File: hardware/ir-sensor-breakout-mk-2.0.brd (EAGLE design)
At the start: 24 x 29 mm, 6 parts, among them U1 MLX906145V-PTH

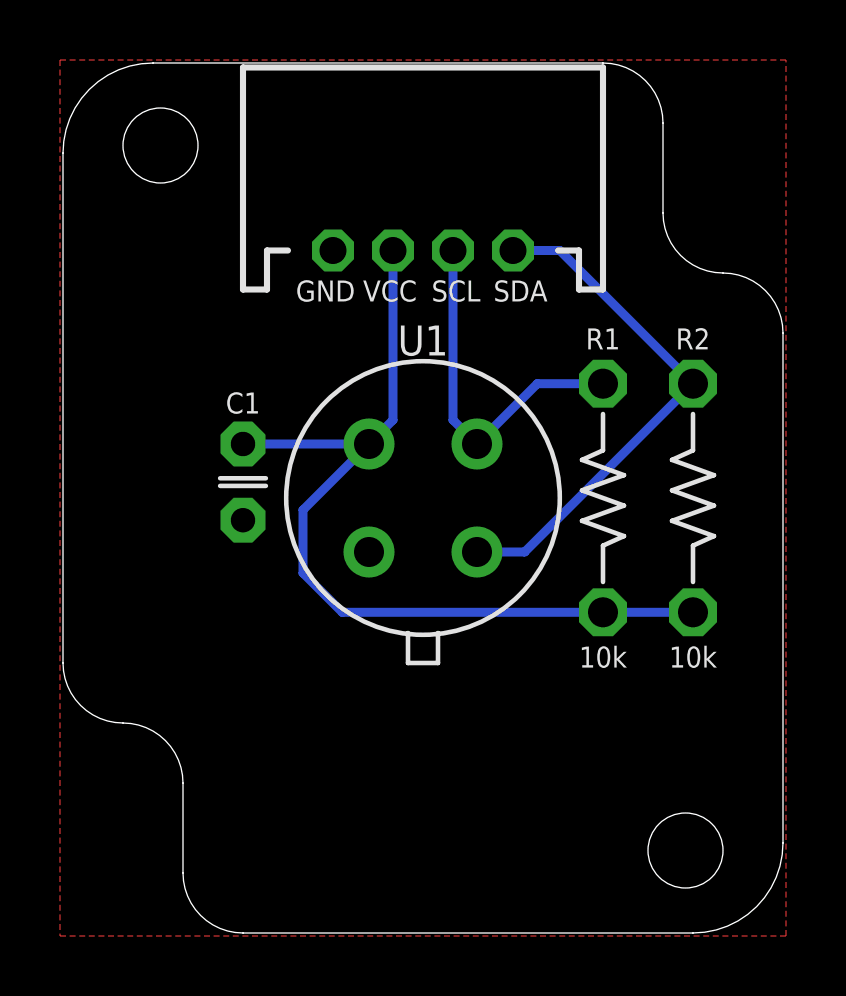
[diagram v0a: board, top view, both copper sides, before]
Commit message: twiddling around with IR sensor breakouts
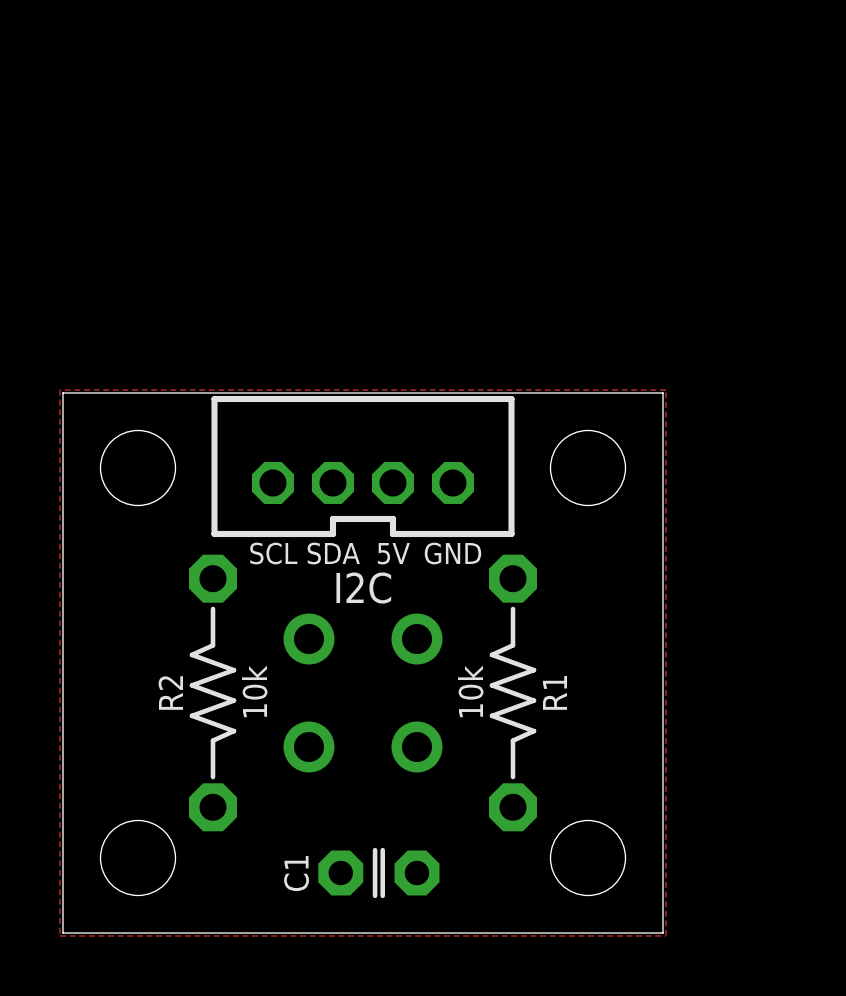
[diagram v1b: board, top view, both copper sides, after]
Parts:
- removed JP1: M04JST-PTH, A_butts:JST-4-PH-RA-PTH
- added I2C: M04JST-PTH-VERT, A_butts:JST-4-PH-VERT-PTH
- C1: value 0.1uF -> 100nF
- FRAME1: value (none) -> FRAME-LETTERNO_PACKAGE
- moved R2 17.3 mm to (5.00, 8.00)
- moved C1 13.8 mm to (10.5, 2.00), turned to 180 degrees
- moved R1 7.16 mm to (15.0, 8.00)
- moved U1 6.80 mm to (10.0, 8.00), flipped to the bottom, turned to 270 degrees
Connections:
- net GND: now also I2C.4; no longer JP1.1
- net SCL: now also I2C.1; no longer JP1.4
- net SDA: now also I2C.2; no longer JP1.3
- net VCC: now also I2C.3; no longer JP1.2
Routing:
- net VCC: track 29.7 -> 0.00 mm
- net SCL: track 17.4 -> 0.00 mm
- net SDA: track 11.8 -> 0.00 mm
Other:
- board size 24 x 29 mm -> 20 x 18 mm
- board text added: "5V"
- board text removed: "VCC"
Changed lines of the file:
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@@
 <board>
 <plain>
-<wire x1="0" y1="26" x2="0" y2="9" width="0" layer="20"/>
-<wire x1="0" y1="9" x2="2" y2="7" width="0" layer="20" curve="90"/>
-<wire x1="2" y1="7" x2="4" y2="5" width="0" layer="20" curve="-90"/>
-<wire x1="4" y1="5" x2="4" y2="2" width="0" layer="20"/>
-<wire x1="4" y1="2" x2="6" y2="0" width="0" layer="20" curve="90"/>
-<wire x1="6" y1="0" x2="21" y2="0" width="0" layer="20"/>
-<wire x1="21" y1="0" x2="24" y2="3" width="0" layer="20" curve="90"/>
-<wire x1="22" y1="22" x2="24" y2="20" width="0" layer="20" curve="-90"/>
-<wire x1="24" y1="20" x2="24" y2="3" width="0" layer="20"/>
-<wire x1="20" y1="27" x2="20" y2="24" width="0" layer="20"/>
-<wire x1="20" y1="24" x2="22" y2="22" width="0" layer="20" curve="90"/>
-<wire x1="20" y1="27" x2="18" y2="29" width="0" layer="20" curve="90"/>
-<wire x1="18" y1="29" x2="3" y2="29" width="0" layer="20"/>
-<wire x1="3" y1="29" x2="0" y2="26" width="0" layer="20" curve="90"/>
-<hole x="20.75" y="2.75" drill="2.5"/>
-<hole x="3.25" y="26.25" drill="2.5"/>
-<text x="8.75" y="21.75" size="0.7" layer="21" font="vector" ratio="12" align="top-center">GND</text>
-<text x="10.9" y="21.75" size="0.7" layer="21" font="vector" ratio="12" align="top-center">VCC</text>
-<text x="15.25" y="21.75" size="0.7" layer="21" font="vector" ratio="12" align="top-center">SDA</text>
-<text x="13.1" y="21.75" size="0.7" layer="21" font="vector" ratio="12" align="top-center">SCL</text>
-<text x="8.75" y="21.75" size="0.7" layer="22" font="vector" ratio="12" rot="MR180" align="bottom-center">GND</text>
-<text x="10.9" y="21.75" size="0.7" layer="22" font="vector" ratio="12" rot="MR180" align="bottom-center">VCC</text>
-<text x="15.25" y="21.75" size="0.7" layer="22" font="vector" ratio="12" rot="MR180" align="bottom-center">SDA</text>
-<text x="13.1" y="21.75" size="0.7" layer="22" font="vector" ratio="12" rot="MR180" align="bottom-center">SCL</text>
+<wire x1="0" y1="18" x2="0" y2="0" width="0" layer="20"/>
+<wire x1="0" y1="0" x2="20" y2="0" width="0" layer="20"/>
+<wire x1="20" y1="18" x2="20" y2="0" width="0" layer="20"/>
+<wire x1="20" y1="18" x2="0" y2="18" width="0" layer="20"/>
+<hole x="17.5" y="15.5" drill="2.5"/>
+<hole x="2.5" y="15.5" drill="2.5"/>
+<text x="13" y="13" size="0.7" layer="21" font="vector" ratio="12" align="top-center">GND</text>
+<text x="11" y="13" size="0.7" layer="21" font="vector" ratio="12" align="top-center">5V</text>
+<text x="9" y="13" size="0.7" layer="21" font="vector" ratio="12" align="top-center">SDA</text>
+<text x="7" y="13" size="0.7" layer="21" font="vector" ratio="12" align="top-center">SCL</text>
+<text x="13" y="13.5" size="0.7" layer="22" font="vector" ratio="12" rot="MR180" align="bottom-center">GND</text>
+<text x="11" y="13.5" size="0.7" layer="22" font="vector" ratio="12" rot="MR180" align="bottom-center">5V</text>
+<text x="9" y="13.5" size="0.7" layer="22" font="vector" ratio="12" rot="MR180" align="bottom-center">SDA</text>
+<text x="7" y="13.5" size="0.7" layer="22" font="vector" ratio="12" rot="MR180" align="bottom-center">SCL</text>
+<hole x="17.5" y="2.5" drill="2.5"/>
+<hole x="2.5" y="2.5" drill="2.5"/>
 </plain>
 <attributes>
@@
 </autorouter>
 <elements>
-<element name="FRAME1" library="A_butts" package="DUMMY" value="" x="0" y="0">
+<element name="FRAME1" library="A_butts" package="DUMMY" value="FRAME-LETTERNO_PACKAGE" x="0" y="0">
 <attribute name="VERSION" value="v01" x="0" y="0" size="0.5" layer="27" font="vector" ratio="12" display="off"/>
 <attribute name="DESIGNER" value="Nobody" x="0" y="0" size="0.5" layer="27" font="vector" ratio="12" display="off"/>
 </element>
-<element name="JP1" library="A_butts" package="JST-4-PH-RA-PTH" value="M04JST-PTH" x="9" y="22.75" smashed="yes">
-<attribute name="SKU" value="PRT-09916" x="9" y="22.75" size="1.778" layer="27" display="off"/>
-</element>
-<element name="U1" library="A_butts" package="TO-39-4" value="MLX906145V-PTH" x="12" y="14.5" smashed="yes" rot="R180">
-<attribute name="NAME" x="12" y="19.25" size="1" layer="25" font="vector" ratio="12" rot="R180" align="top-center"/>
-</element>
-<element name="C1" library="A_butts" package="C025-024X044" value="0.1uF" x="6" y="15.03" rot="R270"/>
-<element name="R1" library="A_butts" package="RESISTOR-AXIAL-PTH-7.62MM" value="10k" x="18" y="14.5" rot="R270"/>
-<element name="R2" library="A_butts" package="RESISTOR-AXIAL-PTH-7.62MM" value="10k" x="21" y="14.5" rot="R270"/>
+<element name="I2C" library="A_butts" package="JST-4-PH-VERT-PTH" value="M04JST-PTH-VERT" x="7" y="15" smashed="yes">
+<attribute name="NAME" x="10" y="12" size="1" layer="25" font="vector" ratio="12" align="top-center"/>
+</element>
+<element name="U1" library="A_butts" package="TO-39-4" value="MLX906145V-PTH" x="10" y="8" smashed="yes" rot="MR270">
+<attribute name="NAME" x="15" y="8" size="1" layer="26" font="vector" ratio="12" rot="MR270" align="top-center"/>
+</element>
+<element name="C1" library="A_butts" package="C025-024X044" value="100nF" x="10.53" y="2" smashed="yes" rot="R180">
+<attribute name="NAME" x="8.184" y="2" size="0.8" layer="25" font="vector" ratio="12" rot="R90" align="bottom-center"/>
+<attribute name="VALUE" x="12.756" y="2" size="0.8" layer="27" font="vector" ratio="12" rot="R270" align="bottom-center"/>
+</element>
+<element name="R1" library="A_butts" package="RESISTOR-AXIAL-PTH-7.62MM" value="10k" x="15" y="8" smashed="yes" rot="R270">
+<attribute name="NAME" x="16" y="8" size="0.8" layer="25" font="vector" ratio="12" rot="R270" align="bottom-center"/>
+<attribute name="VALUE" x="14" y="8" size="0.8" layer="21" font="vector" ratio="12" rot="R270" align="top-center"/>
+</element>
+<element name="R2" library="A_butts" package="RESISTOR-AXIAL-PTH-7.62MM" value="10k" x="5" y="8" smashed="yes" rot="R270">
+<attribute name="NAME" x="4" y="8" size="0.8" layer="25" font="vector" ratio="12" rot="R90" align="bottom-center"/>
+<attribute name="VALUE" x="6" y="8" size="0.8" layer="21" font="vector" ratio="12" rot="R90" align="top-center"/>
+</element>
 </elements>
 <signals>
@@
 <contactref element="R1" pad="P$2"/>
 <contactref element="R2" pad="P$2"/>
-<contactref element="JP1" pad="2"/>
 <contactref element="U1" pad="3"/>
-<wire x1="11" y1="22.75" x2="11" y2="17.1" width="0.3" layer="16"/>
-<wire x1="11" y1="17.1" x2="10.2" y2="16.3" width="0.3" layer="16"/>
-<wire x1="6" y1="16.3" x2="10.2" y2="16.3" width="0.3" layer="16"/>
-<wire x1="10.2" y1="16.3" x2="8" y2="14.1" width="0.3" layer="16"/>
-<wire x1="8" y1="14.1" x2="8" y2="12" width="0.3" layer="16"/>
-<wire x1="8" y1="12" x2="9.31" y2="10.69" width="0.3" layer="16"/>
-<wire x1="9.31" y1="10.69" x2="18" y2="10.69" width="0.3" layer="16"/>
-<wire x1="18" y1="10.69" x2="21" y2="10.69" width="0.3" layer="16"/>
+<contactref element="I2C" pad="3"/>
+<wire x1="11.8" y1="6.2" x2="11" y2="15" width="0" layer="19" extent="1-1"/>
+<wire x1="11.8" y1="2" x2="11.8" y2="6.2" width="0" layer="19" extent="1-1"/>
+<wire x1="15" y1="4.19" x2="11.8" y2="6.2" width="0" layer="19" extent="1-1"/>
+<wire x1="5" y1="4.19" x2="11.8" y2="6.2" width="0" layer="19" extent="1-1"/>
 </signal>
 <signal name="GND">
 <contactref element="C1" pad="2"/>
-<contactref element="JP1" pad="1"/>
 <contactref element="U1" pad="4"/>
 <polygon width="0.1524" layer="1">
 <vertex x="-0.1" y="-0.1"/>
-<vertex x="24.1" y="-0.1"/>
-<vertex x="24.1" y="29.1"/>
-<vertex x="-0.1" y="29.1"/>
+<vertex x="20.1" y="-0.1"/>
+<vertex x="20.1" y="18.1"/>
+<vertex x="-0.1" y="18.1"/>
 </polygon>
+<contactref element="I2C" pad="4"/>
 </signal>
 <signal name="SDA">
-<contactref element="JP1" pad="3"/>
 <contactref element="U1" pad="2"/>
 <contactref element="R1" pad="P$1"/>
-<wire x1="13" y1="22.75" x2="13" y2="17.1" width="0.3" layer="16"/>
-<wire x1="13" y1="17.1" x2="13.8" y2="16.3" width="0.3" layer="16"/>
-<wire x1="13.8" y1="16.3" x2="15.81" y2="18.31" width="0.3" layer="16"/>
-<wire x1="15.81" y1="18.31" x2="18" y2="18.31" width="0.3" layer="16"/>
+<contactref element="I2C" pad="2"/>
+<wire x1="11.8" y1="9.8" x2="15" y2="11.81" width="0" layer="19" extent="1-1"/>
+<wire x1="9" y1="15" x2="11.8" y2="9.8" width="0" layer="19" extent="1-1"/>
 </signal>
 <signal name="SCL">
-<contactref element="JP1" pad="4"/>
 <contactref element="U1" pad="1"/>
 <contactref element="R2" pad="P$1"/>
-<wire x1="15" y1="22.75" x2="16.56" y2="22.75" width="0.3" layer="16"/>
-<wire x1="16.56" y1="22.75" x2="21" y2="18.31" width="0.3" layer="16"/>
-<wire x1="13.8" y1="12.7" x2="15.39" y2="12.7" width="0.3" layer="16"/>
-<wire x1="15.39" y1="12.7" x2="21" y2="18.31" width="0.3" layer="16"/>
+<contactref element="I2C" pad="1"/>
+<wire x1="5" y1="11.81" x2="7" y2="15" width="0" layer="19" extent="1-1"/>
+<wire x1="8.2" y1="9.8" x2="7" y2="15" width="0" layer="19" extent="1-1"/>
 </signal>
 </signals>
